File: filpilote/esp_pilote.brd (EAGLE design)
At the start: 56 x 79 mm, 23 parts, among them IC1 ACS758LCB-050B-PFF-T

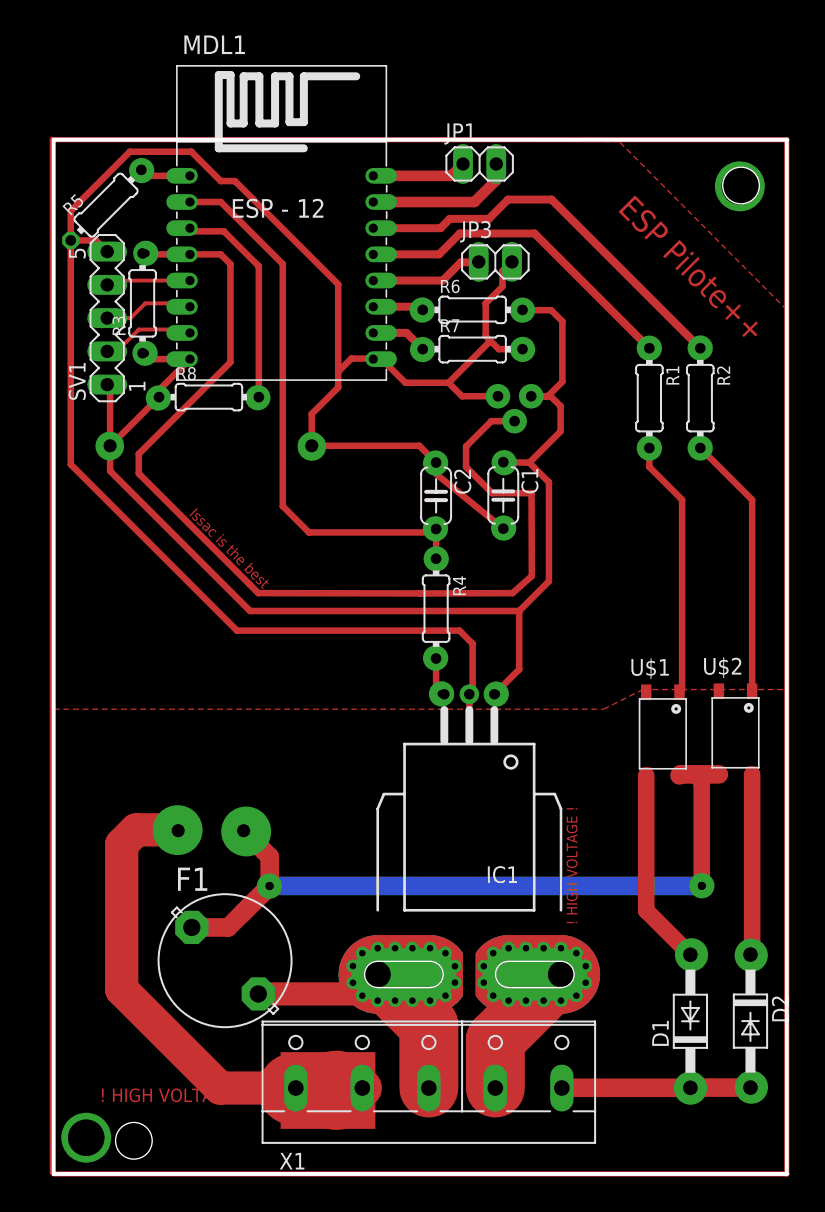
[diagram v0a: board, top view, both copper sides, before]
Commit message: ...
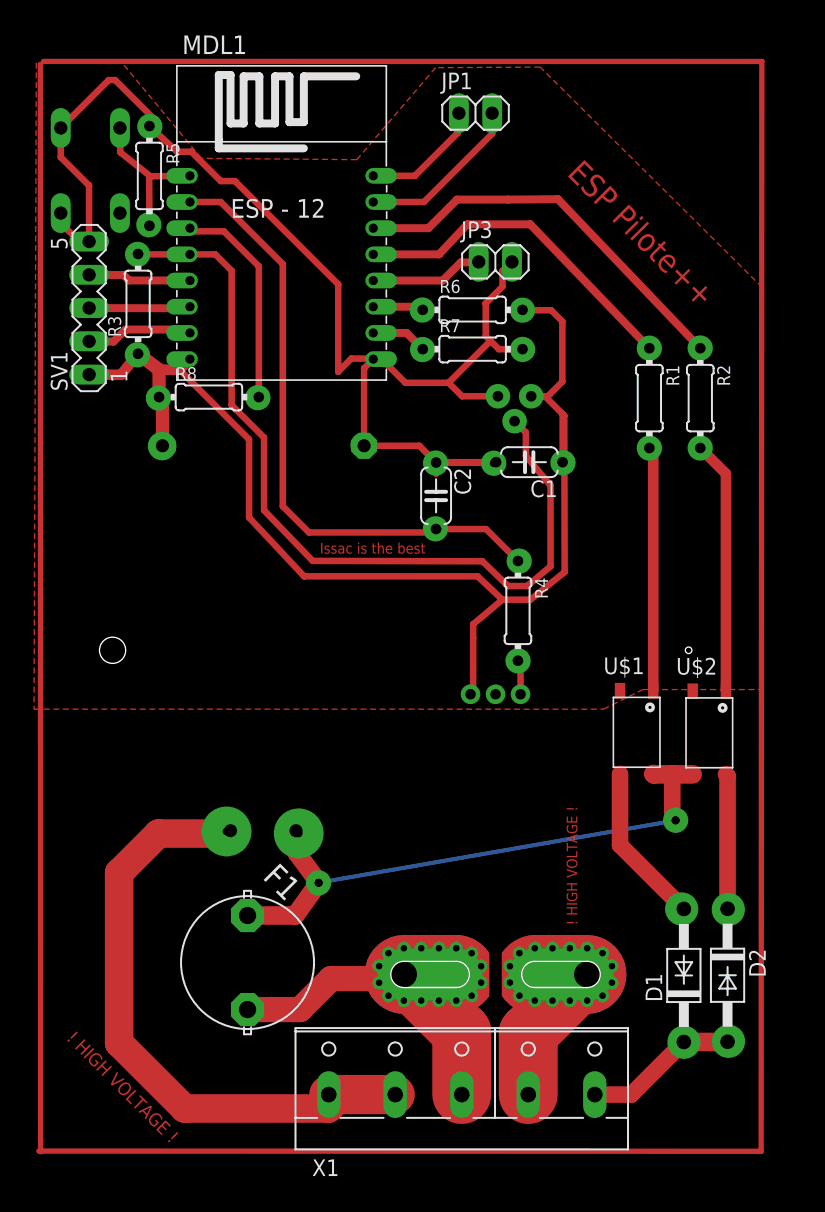
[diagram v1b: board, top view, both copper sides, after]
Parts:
- added S1: (no value), switch-omron:B3F-10XX
- moved R4 6.26 mm to (35.5, 43.0)
- moved U$4 4.00 mm to (16.0, 40.9)
- moved R5 3.99 mm to (7.31, 76.2), turned to 270 degrees
- moved D2 3.91 mm to (51.5, 15.2)
- moved JP1 3.89 mm to (32.2, 81.0)
- moved D1 3.54 mm to (48.1, 15.2)
- moved C1 3.23 mm to (36.3, 54.4), turned to 180 degrees
- moved X1 2.56 mm to (31.2, 6.70)
- moved U$1 2.00 mm to (43.3, 36.9)
- moved IC1 2.00 mm to (33.8, 15.2), flipped to the bottom
- moved U$2 2.00 mm to (48.8, 36.9)
- moved F1 1.72 mm to (14.8, 16.1), turned to 315 degrees
- moved SV1 1.58 mm to (2.71, 66.1)
- moved R3 0.35 mm to (6.45, 66.5)
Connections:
- net 230IN: now also IC1.IP-, IC1.IP-@10, IC1.IP-@11, IC1.IP-@12, IC1.IP-@13, IC1.IP-@14, IC1.IP-@15, IC1.IP-@16, IC1.IP-@17, IC1.IP-@2, IC1.IP-@3, IC1.IP-@4, IC1.IP-@5, IC1.IP-@6, IC1.IP-@7, IC1.IP-@8, IC1.IP-@9; no longer IC1.IP+, IC1.IP+@10, IC1.IP+@11, IC1.IP+@12, IC1.IP+@13, IC1.IP+@14, IC1.IP+@15, IC1.IP+@16, IC1.IP+@17, IC1.IP+@2, IC1.IP+@3, IC1.IP+@4, IC1.IP+@5, IC1.IP+@6, IC1.IP+@7, IC1.IP+@8, IC1.IP+@9
- net 230OUT: now also IC1.IP+, IC1.IP+@10, IC1.IP+@11, IC1.IP+@12, IC1.IP+@13, IC1.IP+@14, IC1.IP+@15, IC1.IP+@16, IC1.IP+@17, IC1.IP+@2, IC1.IP+@3, IC1.IP+@4, IC1.IP+@5, IC1.IP+@6, IC1.IP+@7, IC1.IP+@8, IC1.IP+@9; no longer IC1.IP-, IC1.IP-@10, IC1.IP-@11, IC1.IP-@12, IC1.IP-@13, IC1.IP-@14, IC1.IP-@15, IC1.IP-@16, IC1.IP-@17, IC1.IP-@2, IC1.IP-@3, IC1.IP-@4, IC1.IP-@5, IC1.IP-@6, IC1.IP-@7, IC1.IP-@8, IC1.IP-@9
- net GND: now also S1.3, S1.4
- net N$13: now also S1.2
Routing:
- net GND: track 149.5 -> 102.1 mm, vias 0 -> 5
- net 230FUSED: track 61.6 -> 45.6 mm
- net DS18B20: track 78.5 -> 64.0 mm
- net 230OUT: track 21.5 -> 11.0 mm
- net NEUTRAL: track 37.4 -> 47.4 mm
- net N$13: track 3.90 -> 11.9 mm
- net 230IN: track 31.0 -> 24.1 mm
- net CURRENT: track 42.5 -> 47.5 mm
- net N$53: track 78.9 -> 83.1 mm
- net N$14: track 7.23 -> 11.1 mm
- net N$1: track 13.8 -> 10.3 mm
- net N$15: track 11.3 -> 14.5 mm
- net N$4: track 15.1 -> 12.3 mm
- net PILOTE: track 14.4 -> 11.8 mm
- net N$12: track 191.0 -> 193.3 mm
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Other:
- board size 56 x 79 mm -> 16 x 2 mm
